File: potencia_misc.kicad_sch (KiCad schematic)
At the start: 68 parts, among them J6 ATX-20, M1 Fan, M2 Fan, M3 Fan, Q1 NMOS, Q10 MMBT2222A, Q11 MMBT2222A, Q12 MMBT2222A, Q13 MMBT2222A, Q14 MMBT2907ALT1G, Q15 MMBT2222A, Q16 MMBT2222A, Q17 MMBT2222A, Q18 MMBT2907ALT1G, Q19 MMBT2222A, Q2 NMOS, Q20 MMBT2907ALT1G, Q3 NMOS, Q4 NMOS, Q9 MMBT2907ALT1G, SW3 SW_Push, U8 TPS54302

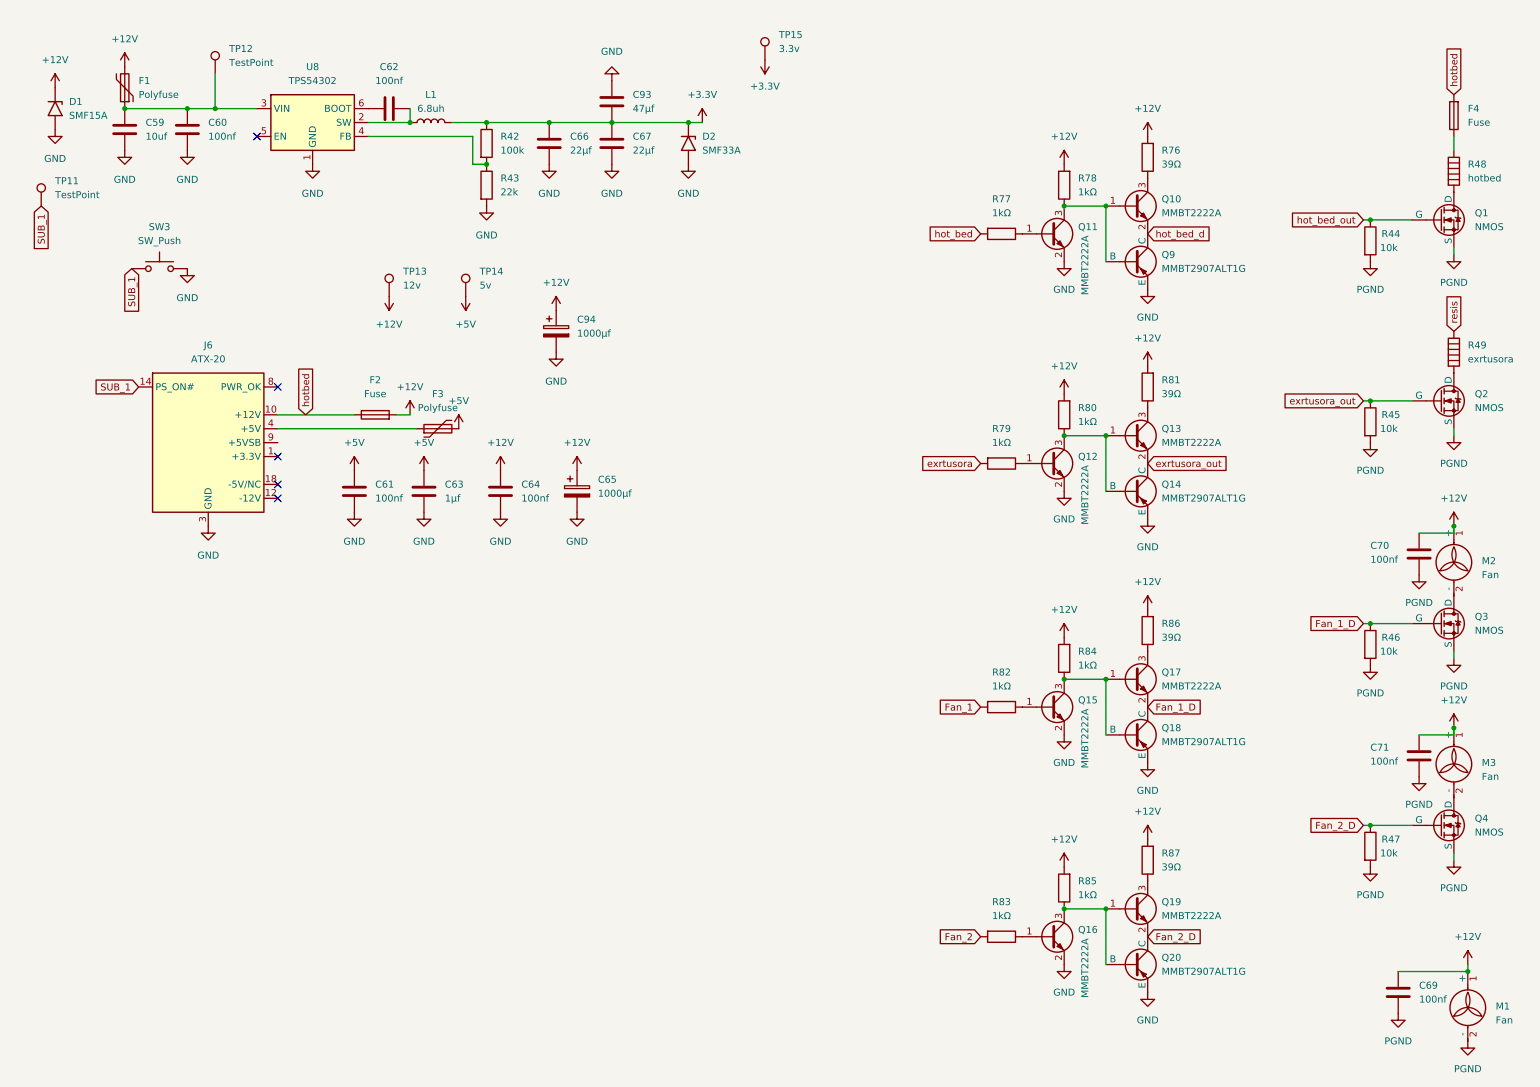
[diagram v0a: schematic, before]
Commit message: 10082026/B
nova revisão
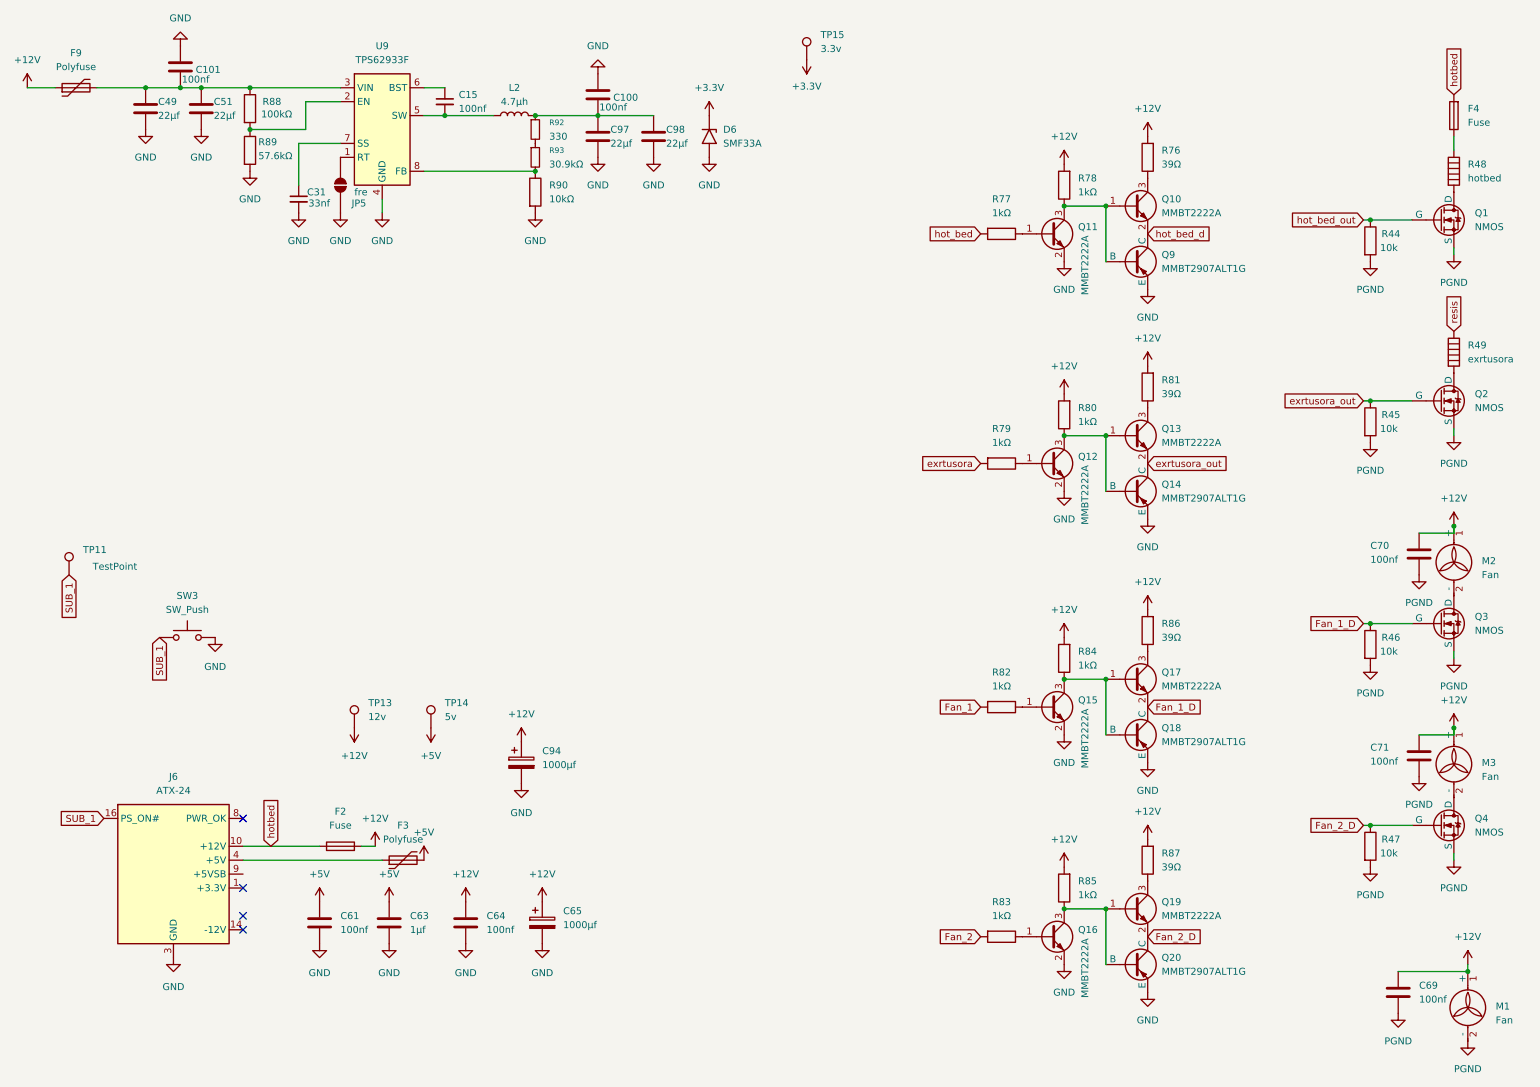
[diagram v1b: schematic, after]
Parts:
- removed C59: 10uf, symbol Device:C
- removed C60, C62: 100nf, Capacitor_SMD:C_0603_1608Metric, symbol Device:C
- removed C66, C67: 22µf, Capacitor_SMD:C_0603_1608Metric, symbol Device:C
- removed C93: 47µf, Capacitor_SMD:C_0603_1608Metric_Pad1.08x0.95mm_HandSolder, symbol Device:C
- removed D1: SMF15A, Diode_SMD:D_SMF, symbol Diode:SMF15A
- removed D2: SMF33A, Diode_SMD:D_SMF, symbol Diode:SMF33A
- removed F1: Polyfuse, symbol Device:Polyfuse
- removed J6: ATX-20, Connector_Molex:Molex_Mini-Fit_Jr_5566-20A_2x10_P4.20mm_Vertical, symbol Connector:ATX-20
- removed L1: 6.8uh, Inductor_SMD:L_Bourns_SRP1038C_10.0x10.0mm, symbol Device:L
- removed R42: 100k, symbol Device:R
- removed R43: 22k, symbol Device:R
- removed TP12: TestPoint, TestPoint:TestPoint_Pad_D1.0mm, symbol Connector:TestPoint
- removed U8: TPS54302, Package_TO_SOT_SMD:SOT-23-6, symbol Regulator_Switching:TPS54302
- added C100, C101: 100nf, Capacitor_SMD:C_0603_1608Metric, symbol Device:C
- added C15: 100nf, symbol Device:C_Small
- added C31: 33nf, Capacitor_SMD:C_0402_1005Metric, symbol Device:C_Small
- added C49, C51, C97, C98: 22µf, symbol Device:C
- added D6: SMF33A, Diode_SMD:D_SMF, symbol Diode:SMF33A
- added F9: Polyfuse, symbol Device:Polyfuse
- added J6: ATX-24, Connector_Molex:Molex_Mini-Fit_Jr_5569-24A2_2x12_P4.20mm_Horizontal, symbol Connector:ATX-24
- added JP5: fre, Jumper:SolderJumper-2_P1.3mm_Open_TrianglePad1.0x1.5mm, symbol Jumper:SolderJumper_2_Open
- added L2: 4.7µh, symbol Device:L
- added R88: 100kΩ, symbol Device:R
- added R89: 57.6kΩ, symbol Device:R
- added R90: 10kΩ, symbol Device:R
- added R92: 330, symbol Device:R_Small
- added R93: 30.9kΩ, symbol Device:R_Small
- added U9: TPS62933F, Package_TO_SOT_SMD:SOT-583-8, symbol Regulator_Switching:TPS62933F
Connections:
- net +12V: now also F9.1
- net +3.3V: now also D6.1 (A1)
- net GND: now also C100.2, C101.2, C31.2, C49.2, C51.2, C97.2, C98.2, D6.2 (A2), J6.15 (GND), J6.17 (GND), J6.18 (GND), J6.19 (GND), J6.24 (GND), J6.3 (GND), J6.5 (GND), J6.7 (GND), JP5.1 (A), R89.2, R90.2, U9.4 (GND)
- net SUB_1: now also J6.16 (PS_ON#)
- net hotbed: now also J6.10 (+12V), J6.11 (+12V)
- net at F3.1: now also J6.21 (+5V), J6.22 (+5V), J6.23 (+5V), J6.4 (+5V), J6.6 (+5V)
- new net: R88.2, R89.1, U9.2 (EN)
- new net: C31.1, U9.7 (SS)
- new net: C15.1, U9.6 (BST)
- new net: C15.2, L2.1, U9.5 (SW)
- new net: C101.1, C49.1, C51.1, F9.2, R88.1, U9.3 (VIN)
- new net: JP5.2 (B), U9.1 (RT)
- new net: R92.2, R93.1
- new net: R90.1, R93.2, U9.8 (FB)
- new net: C100.1, C97.1, C98.1, L2.2, R92.1
- new net: J6.1 (+3.3V), J6.12 (+3.3V), J6.13 (+3.3V), J6.2 (+3.3V)
- no-connect marks 5 -> 4
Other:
- company: (none) -> ---
- moved on the sheet: C61, C63, C64, C65, C94, F2, F3, SW3, TP11, TP13, TP14, TP15
